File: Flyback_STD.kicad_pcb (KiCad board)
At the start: 2 copper layers, 60.6 x 27.5 mm, 103 parts, among them P1 VIN, P2 GND, P3 VOUT, P4 PGND, Q1 HY1420C2, U1 VPC2188B

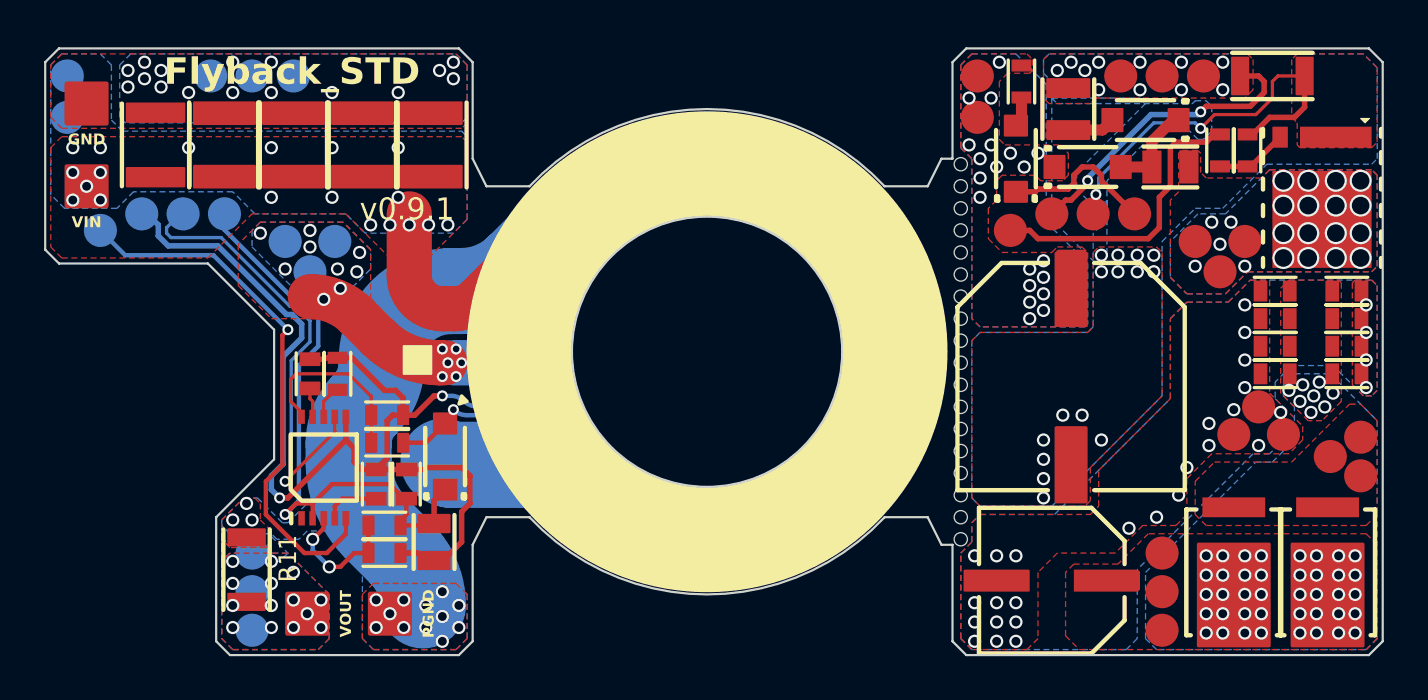
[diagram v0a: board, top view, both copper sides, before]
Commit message: Create new layout
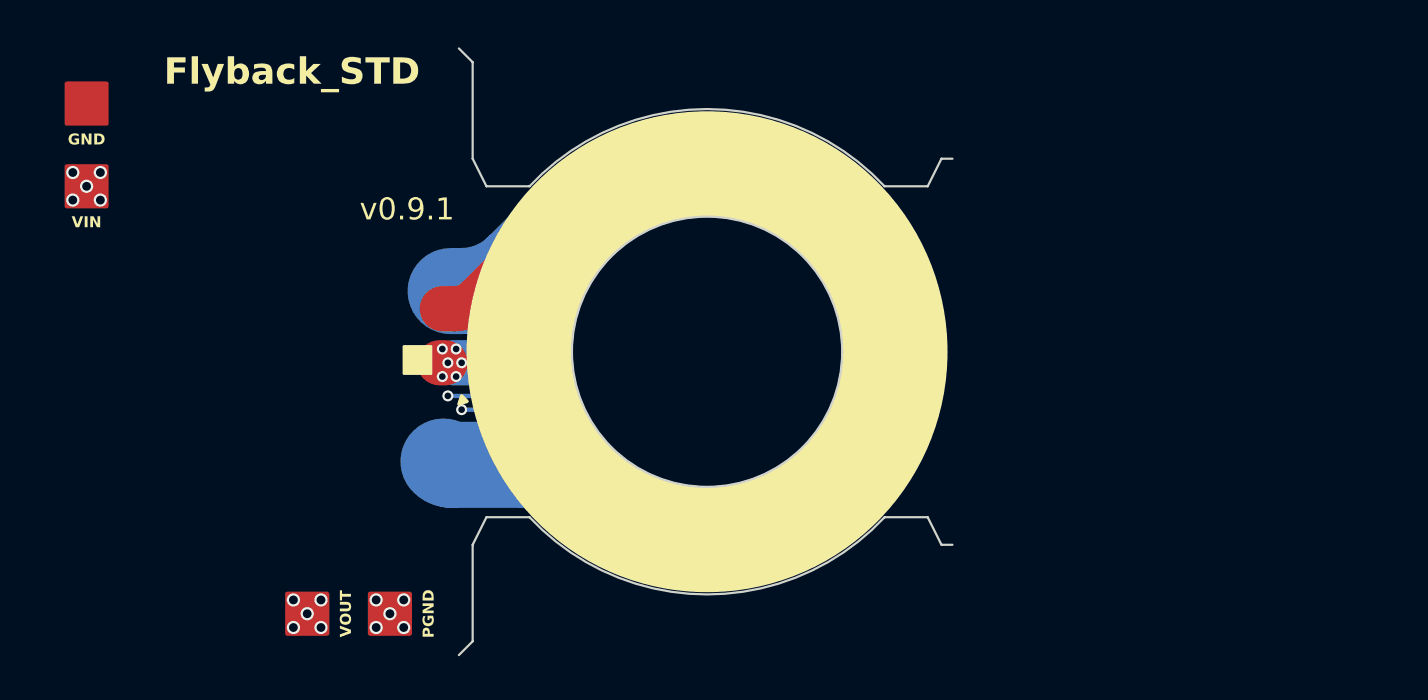
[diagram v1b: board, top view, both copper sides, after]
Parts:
- removed C1, C2: 100nF, 001_GN_RCL_SMD:C0603(1608M)
- removed C10: 10uF, 001_GN_RCL_SMD:C0805(2012M)
- removed C11: 120uF, 007_GN_POLAR-CAP_SMD:CL-0608
- removed C12, C13, C14, C15, C16, C17, C18, C19: 10uF, 001_GN_RCL_SMD:C0603(1608M)
- removed C3: 1nF, 001_GN_RCL_SMD:C0603(1608M)
- removed C4, C5, C6, C7: 4.7uF, 001_GN_RCL_SMD:C1210(3225M)
- removed C8: 100uF, 007_GN_POLAR-CAP_SMD:CL-1010
- removed C9: 1nF, 001_GN_RCL_SMD:C0805(2012M)
- removed D1, D4: DS110W, 002_GN_TWO-PIN_PLASTIC_SMD:SOD-123F
- removed D2, D3: DS120W, 002_GN_TWO-PIN_PLASTIC_SMD:SOD-123F
- removed D5, D6: SB2080L, 102_SP_POWER_DIODE_SMD:TO-277B
- removed L1: 1uH, 008_GN_POWER-CHOKE_SMD:MC-2520
- removed Q1: HY1420C2, 103_SP_POWER_TRANSISTOR_SMD:SON-FET_6050
- removed R1: 100R, 001_GN_RCL_SMD:R0603(1608M)
- removed R10: 3.9k, 001_GN_RCL_SMD:R0603(1608M)
- removed R11: 2.2k, 001_GN_RCL_SMD:R1206(3216M)
- removed R2: 100k, 001_GN_RCL_SMD:R0603(1608M)
- removed R3: 5.6k, 001_GN_RCL_SMD:R0603(1608M)
- removed R4: 27k, 001_GN_RCL_SMD:R0603(1608M)
- removed R5: RL1210A680K, 001_GN_RCL_SMD:R1210(3225M)
- removed R6: 2.2R, 001_GN_RCL_SMD:R0603(1608M)
- removed R7: 10k, 001_GN_RCL_SMD:R0603(1608M)
- removed R8: 25mR/1W, 001_GN_RCL_SMD:R1206(3216M)
- removed R9: 36k, 001_GN_RCL_SMD:R0603(1608M)
- removed REF** (x18): NPTH-C_1006, 302_MECH_PAD:NPTH-C_1006
- removed REF** (x42): SMP-C_15, 302_MECH_PAD:SMP-C_15
- removed U1: VPC2188B, 004_GN_MIDDLE-SEMI_SMD:MSOP-10_3030
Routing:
- net GND: track 117.3 -> 52.2 mm, vias 47 -> 2
- net /CS: track 39.1 -> 0.00 mm, vias 3 -> 0
- net /GT_U: track 38.0 -> 0.00 mm, vias 1 -> 0
- net VDD: track 34.9 -> 0.00 mm, vias 1 -> 0
- net GNDPWR: track 70.6 -> 53.2 mm, vias 44 -> 5
- net VBUS: track 121.1 -> 109.2 mm, vias 81 -> 17
- net Net-(U1-FB): track 8.19 -> 0.00 mm
- net /UVP: track 6.00 -> 0.00 mm, vias 2 -> 0
- net Net-(D2-Anode): track 4.19 -> 0.00 mm
- net /GT: track 3.27 -> 0.00 mm
- net Vdrive: track 2.56 -> 0.00 mm
- net Net-(D3-Anode): track 2.19 -> 0.00 mm
- net /RT: track 1.54 -> 0.00 mm
- net Net-(D1-Anode): track 1.38 -> 0.00 mm
- net /SS: track 1.34 -> 0.00 mm
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- removed copper zone on F.Cu, net /CS
- removed copper zone on B.Cu, net GND
- removed copper zone on F.Cu, net GND
- removed copper zone on B.Cu, net GNDPWR
- removed copper zone on F.Cu, net GNDPWR
- removed copper zone on B.Cu, net VBUS
- removed copper zone on F.Cu, net VBUS
- removed copper zone on B.Cu, net VDC
- removed copper zone on F.Cu, net VDC
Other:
- board size 60.6 x 27.5 mm -> 22.4 x 27.5 mm
- board text removed: "PkgLAN"

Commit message: Nightly update
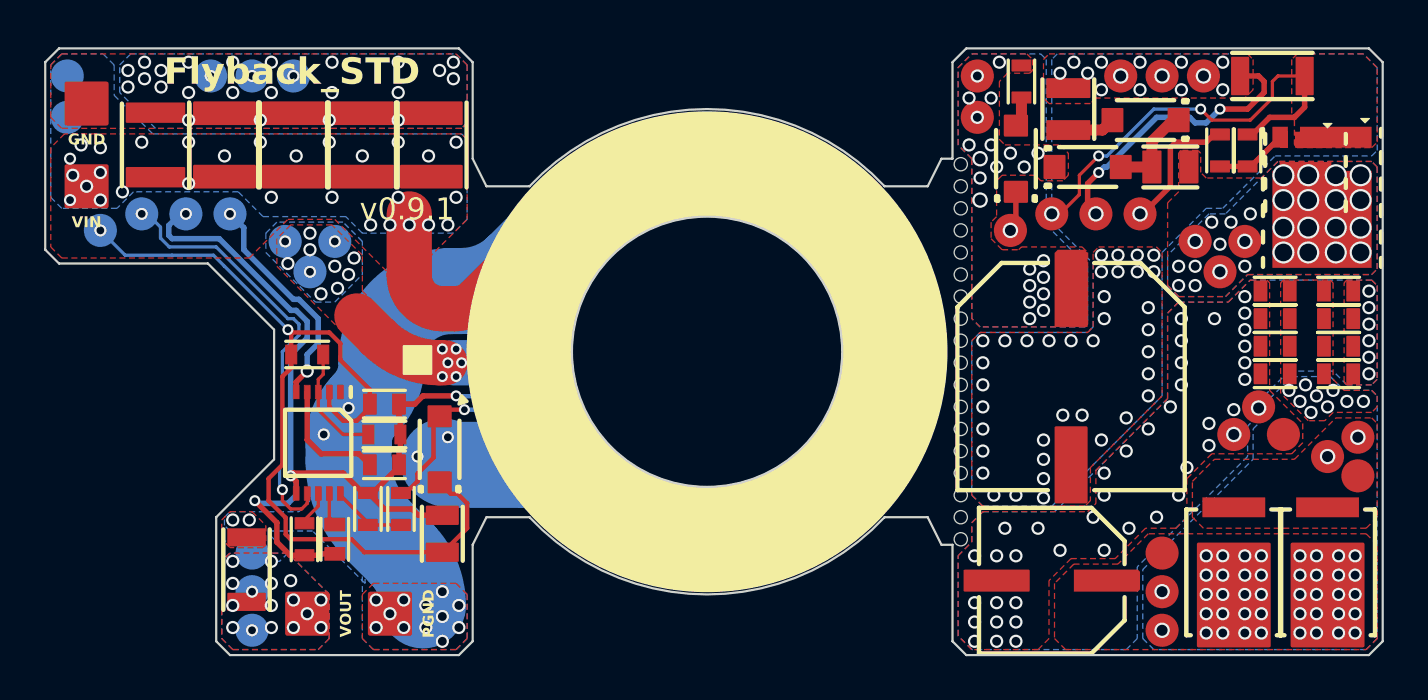
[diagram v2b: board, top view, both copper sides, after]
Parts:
- added C1: 100nF, 001_GN_RCL_SMD:C0603(1608M), F.Cu at (85.4, 105.1)
- added C10: 10uF, 001_GN_RCL_SMD:C0805(2012M), F.Cu at (88.0, 108.2)
- added C11: 120uF, 007_GN_POLAR-CAP_SMD:CL-0608, F.Cu at (115.6, 110.4)
- added C12: 10uF, 001_GN_RCL_SMD:C0603(1608M), F.Cu at (125.8, 97.2)
- added C13: 10uF, 001_GN_RCL_SMD:C0603(1608M), F.Cu at (128.6, 97.2)
- added C14: 10uF, 001_GN_RCL_SMD:C0603(1608M), F.Cu at (125.8, 98.5)
- added C15: 10uF, 001_GN_RCL_SMD:C0603(1608M), F.Cu at (128.6, 98.5)
- added C16: 10uF, 001_GN_RCL_SMD:C0603(1608M), F.Cu at (125.8, 99.8)
- added C17: 10uF, 001_GN_RCL_SMD:C0603(1608M), F.Cu at (128.6, 99.8)
- added C18: 10uF, 001_GN_RCL_SMD:C0603(1608M), F.Cu at (125.8, 101.0)
- added C19: 10uF, 001_GN_RCL_SMD:C0603(1608M), F.Cu at (128.6, 101.0)
- added C2: 100nF, 001_GN_RCL_SMD:C0603(1608M), F.Cu at (85.4, 102.4)
- added C3: 1nF, 001_GN_RCL_SMD:C0603(1608M), F.Cu at (83.1, 108.5)
- added C4: 4.7uF, 001_GN_RCL_SMD:C1210(3225M), F.Cu at (78.1, 90.6)
- added C5: 4.7uF, 001_GN_RCL_SMD:C1210(3225M), F.Cu at (81.2, 90.6)
- added C6: 4.7uF, 001_GN_RCL_SMD:C1210(3225M), F.Cu at (84.4, 90.6)
- added C7: 4.7uF, 001_GN_RCL_SMD:C1210(3225M), F.Cu at (87.5, 90.6)
- added C8: 100uF, 007_GN_POLAR-CAP_SMD:CL-1010, F.Cu at (116.5, 101.1)
- added C9: 1nF, 001_GN_RCL_SMD:C0805(2012M), F.Cu at (121.0, 91.6)
- added D1: DS110W, 002_GN_TWO-PIN_PLASTIC_SMD:SOD-123F, F.Cu at (114.0, 91.2)
- added D2: DS120W, 002_GN_TWO-PIN_PLASTIC_SMD:SOD-123F, F.Cu at (117.2, 91.6)
- added D3: DS120W, 002_GN_TWO-PIN_PLASTIC_SMD:SOD-123F, F.Cu at (119.9, 89.5)
- added D4: DS110W, 002_GN_TWO-PIN_PLASTIC_SMD:SOD-123F, F.Cu at (87.9, 104.4)
- added D5: SB2080L, 102_SP_POWER_DIODE_SMD:TO-277B, F.Cu at (128.1, 110.0)
- added D6: SB2080L, 102_SP_POWER_DIODE_SMD:TO-277B, F.Cu at (123.9, 110.0)
- added L1: 10uH, 008_GN_POWER-CHOKE_SMD:MC-2520, F.Cu at (116.4, 89.0)
- added Q1: HY1420C2, 103_SP_POWER_TRANSISTOR_SMD:SON-FET_6050, F.Cu at (127.9, 93.0)
- added Q2: HSBB0012, 103_SP_POWER_TRANSISTOR_SMD:SON-FET_3333, F.Cu at (127.1, 91.9)
- added R1: 100R, 001_GN_RCL_SMD:R0603(1608M), F.Cu at (114.2, 87.8)
- added R10: 3.9k, 001_GN_RCL_SMD:R0603(1608M), F.Cu at (84.6, 107.1)
- added R11: 2.2k, 001_GN_RCL_SMD:R1206(3216M), F.Cu at (79.1, 109.9)
- added R2: 100k, 001_GN_RCL_SMD:R0603(1608M), F.Cu at (81.9, 100.1)
- added R3: 5.6k, 001_GN_RCL_SMD:R0603(1608M), F.Cu at (85.4, 103.8)
- added R4: 27k, 001_GN_RCL_SMD:R0603(1608M), F.Cu at (81.8, 108.5)
- added R5: RL1210A680K, 001_GN_RCL_SMD:R1210(3225M), F.Cu at (75.0, 90.6)
- added R6: 2.2R, 001_GN_RCL_SMD:R0603(1608M), F.Cu at (123.2, 90.9)
- added R7: 10k, 001_GN_RCL_SMD:R0603(1608M), F.Cu at (124.5, 90.9)
- added R8: 25mR/1W, 001_GN_RCL_SMD:R1206(3216M), F.Cu at (125.6, 87.5)
- added R9: 33k, 001_GN_RCL_SMD:R0603(1608M), F.Cu at (86.1, 107.1)
- added REF**: NPTH-C_1006, 302_MECH_PAD:NPTH-C_1006, F.Cu at (111.5, 96.5)
- added REF**: NPTH-C_1006, 302_MECH_PAD:NPTH-C_1006, F.Cu at (111.5, 99.5)
- added REF**: SMP-C_15, 302_MECH_PAD:SMP-C_15, F.Cu at (128.1, 104.8)
- added REF**: NPTH-C_1006, 302_MECH_PAD:NPTH-C_1006, F.Cu at (111.5, 101.5)
- added REF**: NPTH-C_1006, 302_MECH_PAD:NPTH-C_1006, F.Cu at (111.5, 91.5)
- added REF**: SMP-C_15, 302_MECH_PAD:SMP-C_15, F.Cu at (120.6, 110.9)
- added REF**: NPTH-C_1006, 302_MECH_PAD:NPTH-C_1006, F.Cu at (111.5, 108.5)
- added REF**: SMP-C_15, 302_MECH_PAD:SMP-C_15, F.Cu at (129.5, 103.9)
- added REF**: SMP-C_15, 302_MECH_PAD:SMP-C_15, F.Cu at (123.2, 96.4)
- added REF**: SMP-C_15, 302_MECH_PAD:SMP-C_15, F.Cu at (113.8, 94.5)
- added REF**: SMP-C_15, 302_MECH_PAD:SMP-C_15, F.Cu at (124.4, 95.0)
- added REF**: SMP-C_15, 302_MECH_PAD:SMP-C_15, F.Cu at (123.9, 103.8)
- added REF**: SMP-C_15, 302_MECH_PAD:SMP-C_15, F.Cu at (125.0, 102.5)
- added REF**: SMP-C_15, 302_MECH_PAD:SMP-C_15, F.Cu at (112.2, 89.4)
- added REF**: SMP-C_15, 302_MECH_PAD:SMP-C_15, F.Cu at (119.6, 93.8)
- added REF**: NPTH-C_1006, 302_MECH_PAD:NPTH-C_1006, F.Cu at (111.5, 93.5)
- added REF**: NPTH-C_1006, 302_MECH_PAD:NPTH-C_1006, F.Cu at (111.5, 104.5)
- added REF**: SMP-C_15, 302_MECH_PAD:SMP-C_15, F.Cu at (120.6, 109.1)
- added REF**: SMP-C_15, 302_MECH_PAD:SMP-C_15, F.Cu at (112.2, 87.5)
- added REF**: SMP-C_15, 302_MECH_PAD:SMP-C_15, F.Cu at (120.6, 112.6)
- added REF**: SMP-C_15, 302_MECH_PAD:SMP-C_15, F.Cu at (122.1, 95.0)
- added REF**: NPTH-C_1006, 302_MECH_PAD:NPTH-C_1006, F.Cu at (111.5, 107.5)
- added REF**: NPTH-C_1006, 302_MECH_PAD:NPTH-C_1006, F.Cu at (111.5, 94.5)
- added REF**: SMP-C_15, 302_MECH_PAD:SMP-C_15, F.Cu at (115.6, 93.8)
- added REF**: NPTH-C_1006, 302_MECH_PAD:NPTH-C_1006, F.Cu at (111.5, 95.5)
- added REF**: NPTH-C_1006, 302_MECH_PAD:NPTH-C_1006, F.Cu at (111.5, 106.5)
- added REF**: NPTH-C_1006, 302_MECH_PAD:NPTH-C_1006, F.Cu at (111.5, 103.5)
- added REF**: NPTH-C_1006, 302_MECH_PAD:NPTH-C_1006, F.Cu at (111.5, 97.5)
- added REF**: SMP-C_15, 302_MECH_PAD:SMP-C_15, F.Cu at (126.1, 103.8)
- added REF**: NPTH-C_1006, 302_MECH_PAD:NPTH-C_1006, F.Cu at (111.5, 92.5)
- added REF**: SMP-C_15, 302_MECH_PAD:SMP-C_15, F.Cu at (117.6, 93.8)
- added REF**: NPTH-C_1006, 302_MECH_PAD:NPTH-C_1006, F.Cu at (111.5, 98.5)
- added REF**: SMP-C_15, 302_MECH_PAD:SMP-C_15, F.Cu at (122.5, 87.5)
- added REF**: NPTH-C_1006, 302_MECH_PAD:NPTH-C_1006, F.Cu at (111.5, 102.5)
- added REF**: SMP-C_15, 302_MECH_PAD:SMP-C_15, B.Cu at (77.5, 87.5)
- added REF**: SMP-C_15, 302_MECH_PAD:SMP-C_15, B.Cu at (79.4, 110.9)
- added REF**: SMP-C_15, 302_MECH_PAD:SMP-C_15, B.Cu at (82.0, 96.4)
- added REF**: SMP-C_15, 302_MECH_PAD:SMP-C_15, B.Cu at (76.4, 93.8)
- added REF**: SMP-C_15, 302_MECH_PAD:SMP-C_15, B.Cu at (71.0, 89.4)
- added REF**: SMP-C_15, 302_MECH_PAD:SMP-C_15, B.Cu at (79.4, 87.5)
- added REF**: SMP-C_15, 302_MECH_PAD:SMP-C_15, B.Cu at (79.4, 109.1)
- added REF**: SMP-C_15, 302_MECH_PAD:SMP-C_15, B.Cu at (80.9, 95.0)
- added REF**: SMP-C_15, 302_MECH_PAD:SMP-C_15, B.Cu at (84.9, 103.8)
- added REF**: SMP-C_15, 302_MECH_PAD:SMP-C_15, B.Cu at (74.4, 93.8)
- added REF**: SMP-C_15, 302_MECH_PAD:SMP-C_15, F.Cu at (120.6, 87.5)
- added REF**: SMP-C_15, 302_MECH_PAD:SMP-C_15, B.Cu at (72.5, 94.5)
- added REF**: SMP-C_15, 302_MECH_PAD:SMP-C_15, B.Cu at (81.2, 87.5)
- added REF**: SMP-C_15, 302_MECH_PAD:SMP-C_15, B.Cu at (86.9, 104.8)
- added REF**: SMP-C_15, 302_MECH_PAD:SMP-C_15, B.Cu at (79.4, 112.6)
- added REF**: SMP-C_15, 302_MECH_PAD:SMP-C_15, B.Cu at (83.8, 102.5)
- added REF**: SMP-C_15, 302_MECH_PAD:SMP-C_15, B.Cu at (78.4, 93.8)
- added REF**: SMP-C_15, 302_MECH_PAD:SMP-C_15, B.Cu at (71.0, 87.5)
- added REF**: SMP-C_15, 302_MECH_PAD:SMP-C_15, B.Cu at (83.1, 95.0)
- added REF**: SMP-C_15, 302_MECH_PAD:SMP-C_15, B.Cu at (88.2, 105.6)
- added REF**: SMP-C_15, 302_MECH_PAD:SMP-C_15, B.Cu at (82.6, 103.8)
- added REF**: SMP-C_15, 302_MECH_PAD:SMP-C_15, F.Cu at (129.5, 105.6)
- added REF**: SMP-C_15, 302_MECH_PAD:SMP-C_15, B.Cu at (88.2, 103.9)
- added REF**: SMP-C_15, 302_MECH_PAD:SMP-C_15, F.Cu at (118.8, 87.5)
- added REF**: NPTH-C_1006, 302_MECH_PAD:NPTH-C_1006, F.Cu at (111.5, 100.5)
- added REF**: NPTH-C_1006, 302_MECH_PAD:NPTH-C_1006, F.Cu at (111.5, 105.5)
- added U1: VPC2188B, 004_GN_MIDDLE-SEMI_SMD:MSOP-10_3030, F.Cu at (82.4, 104.1)
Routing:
- net GND: track 52.2 -> 111.5 mm, vias 2 -> 85
- net VDD: track 0.00 -> 43.2 mm, vias 0 -> 3
- net /CS: track 0.00 -> 39.7 mm, vias 0 -> 5
- net GNDPWR: track 53.2 -> 70.6 mm, vias 5 -> 68
- net /GT_U: track 0.00 -> 16.4 mm, vias 0 -> 3
- net VBUS: track 109.2 -> 118.7 mm, vias 17 -> 102
- net Vdrive: track 0.00 -> 5.48 mm
- net /UVP: track 0.00 -> 5.33 mm
- net Net-(D2-Anode): track 0.00 -> 4.19 mm
- net Net-(U1-FB): track 0.00 -> 3.44 mm
- net /GT: track 0.00 -> 3.27 mm
- net Net-(D3-Anode): track 0.00 -> 2.19 mm
- net /RT: track 0.00 -> 1.61 mm
- net /SS: track 0.00 -> 1.52 mm
- net Net-(D1-Anode): track 0.00 -> 1.38 mm
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- added copper zone on F.Cu, net /CS
- added copper zone on B.Cu, net GND
- added copper zone on F.Cu, net GND
- added copper zone on B.Cu, net GNDPWR
- added copper zone on F.Cu, net GNDPWR
- added copper zone on B.Cu, net VBUS
- added copper zone on F.Cu, net VBUS
- added copper zone on B.Cu, net VDC
- added copper zone on F.Cu, net VDC
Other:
- board size 22.4 x 27.5 mm -> 60.6 x 27.5 mm
- board text added: "PkgLAN"
